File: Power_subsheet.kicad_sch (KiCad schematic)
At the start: 29 parts, among them U3 LM1117MP-ADJ, U4 TPS54331QDRQ1

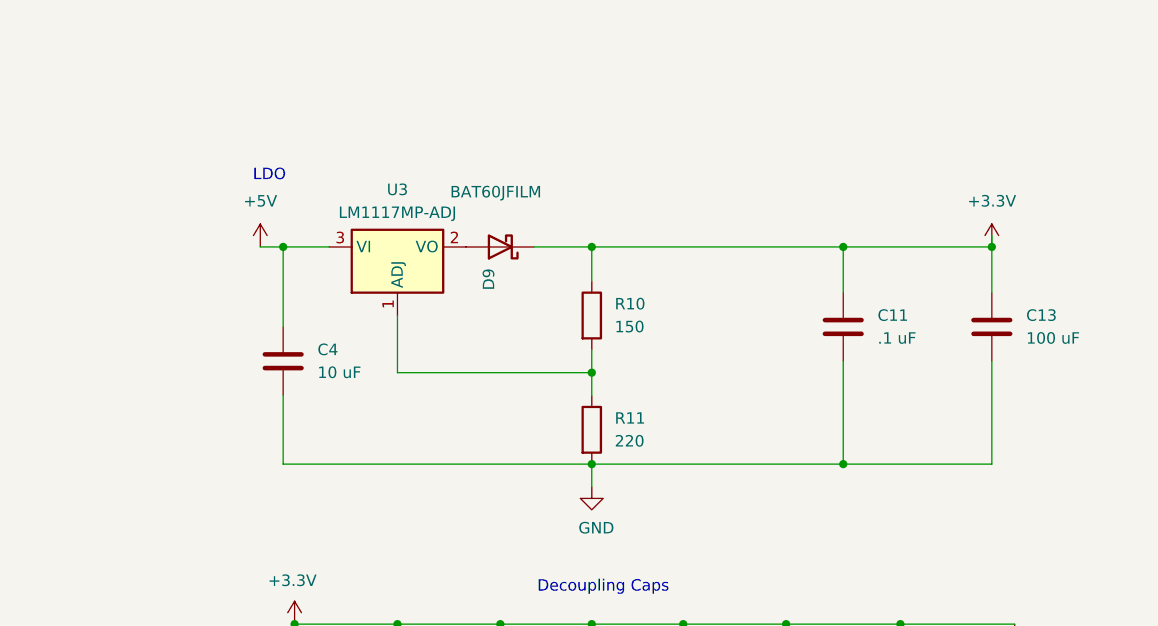
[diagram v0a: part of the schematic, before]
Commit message: changes
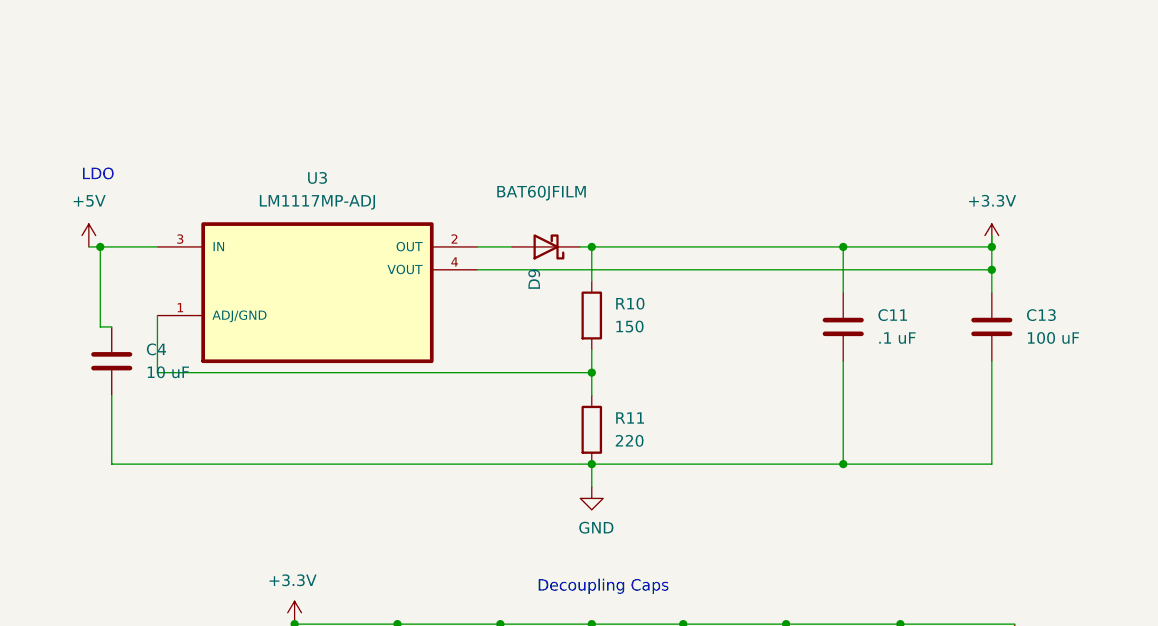
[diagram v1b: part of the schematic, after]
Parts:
- removed U3: LM1117MP-ADJ, Package_TO_SOT_SMD:SOT-223, symbol Regulator_Linear:LM1117MP-ADJ
- added U3: LM1117MP-ADJ, Library:REALWORKLDOFT, symbol New_Library:LM1117MP-ADJ
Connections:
- net +3.3V: now also U3.4 (VOUT)
- net +5V: now also U3.3 (IN)
- net at R10.2, R11.1: now also U3.1 (ADJ/GND)
- net at D9.2 (A): now also U3.2 (OUT)
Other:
- moved on the sheet: C4, D9
